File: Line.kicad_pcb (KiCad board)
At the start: 2 copper layers, 141 x 29 mm, 50 parts, among them U0 QRE1113GR, U1 QRE1113GR, U10 QRE1113GR, U11 QRE1113GR, U12 QRE1113GR, U13 QRE1113GR, U14 QRE1113GR, U16 CD74HC4067M, U2 QRE1113GR, U3 QRE1113GR, U4 QRE1113GR, U5 QRE1113GR, U6 QRE1113GR, U7 QRE1113GR, U8 QRE1113GR, U9 QRE1113GR

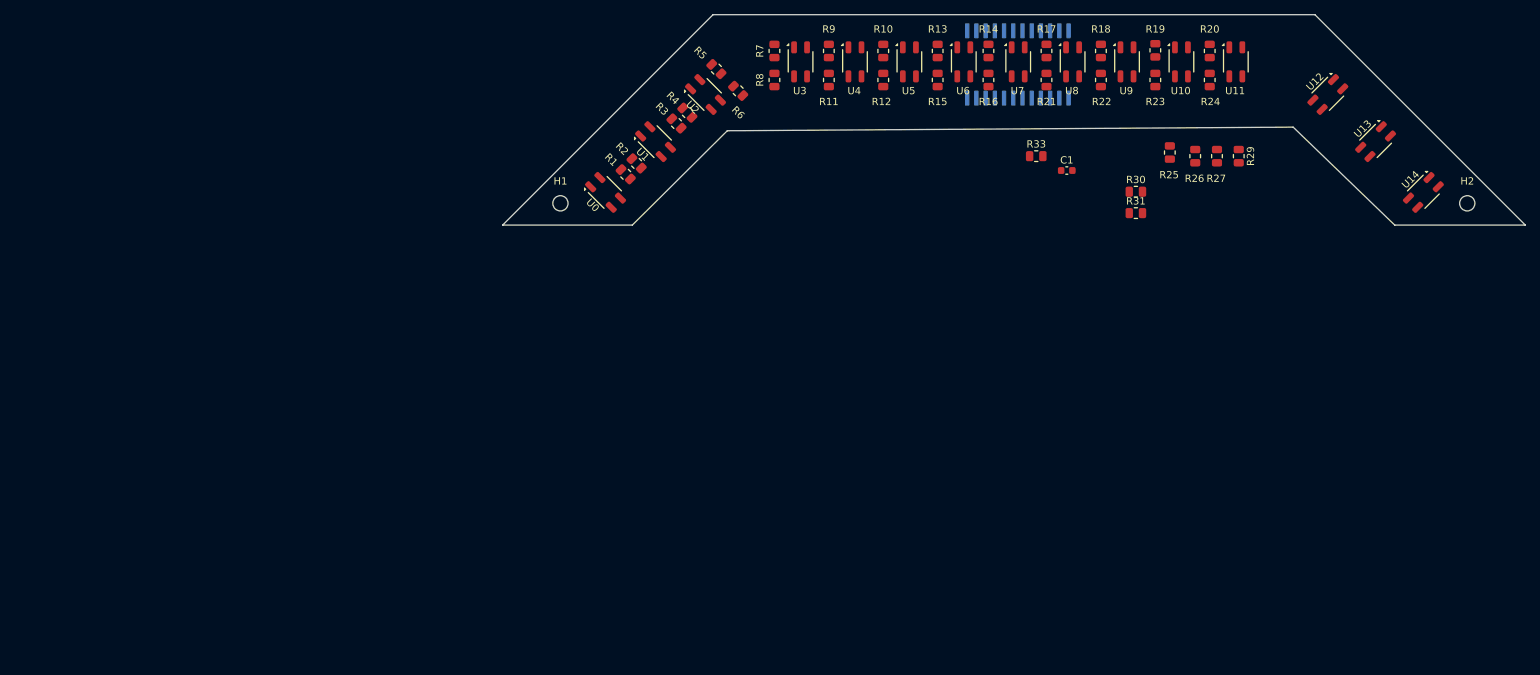
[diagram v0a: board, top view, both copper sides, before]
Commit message: sap route
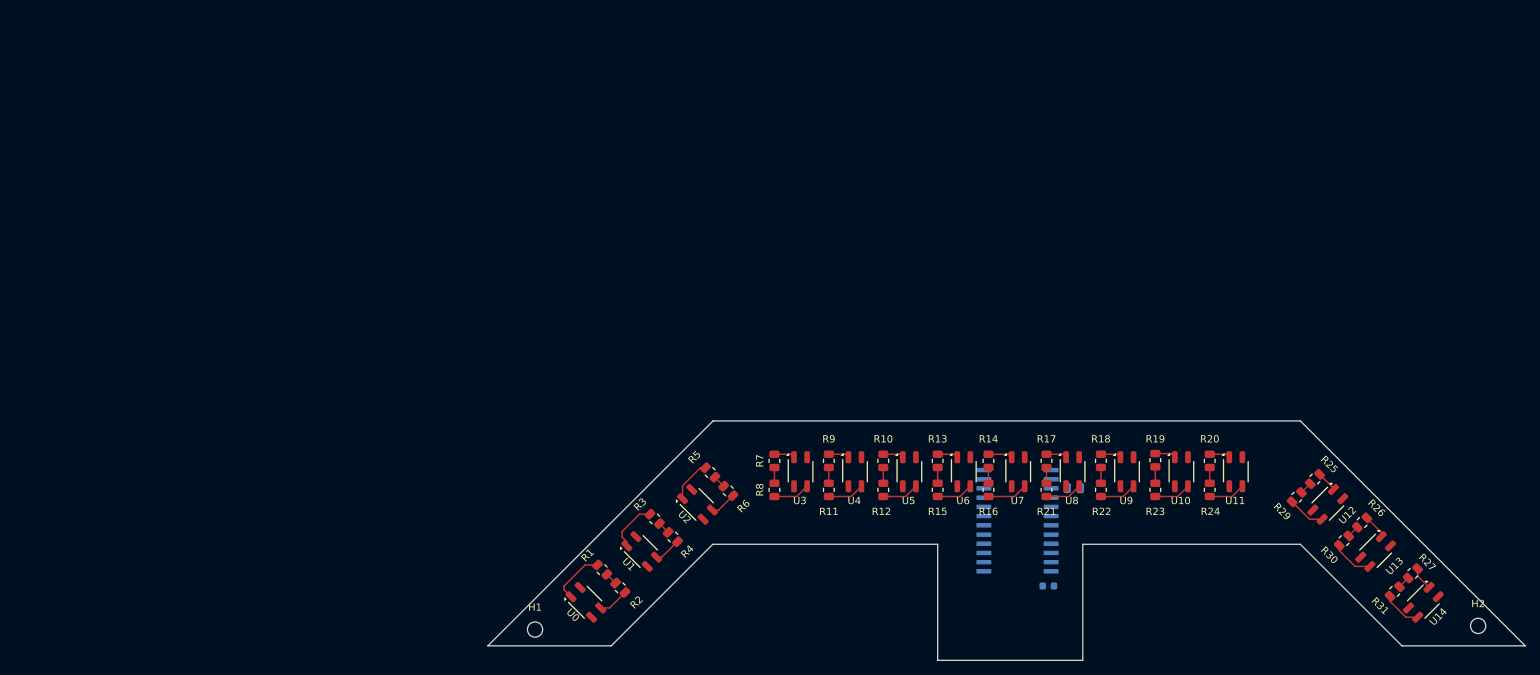
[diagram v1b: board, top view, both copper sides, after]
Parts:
- C1, R33: moved to B.Cu
- moved R27 63.5 mm to (267.0, 142.0), turned to 45 degrees
- moved R31 63.2 mm to (264.5, 144.5), turned to -135 degrees
- moved U16 62.9 mm to (212.5, 134.8), turned to 0 degrees
- moved H1 58.9 mm to (146.0, 149.8)
- moved R2 58.5 mm to (157.8, 144.0), turned to -45 degrees
- moved R4 58.5 mm to (165.0, 137.0), turned to -45 degrees
- moved H2 58.3 mm to (276.0, 149.2)
- moved C1 57.3 mm to (216.8, 143.8), turned to 180 degrees
- moved U0 56.6 mm to (153.0, 146.0)
- moved U1 56.5 mm to (160.7, 139.0)
- moved U2 56.5 mm to (168.4, 132.5)
- moved R10 56.5 mm to (194.0, 126.5)
- moved R11 56.5 mm to (186.5, 130.5)
- moved R12 56.5 mm to (194.0, 130.5)
- moved R13 56.5 mm to (201.5, 126.5)
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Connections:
- U1 pad 1: Net-(U0-A) -> Net-(U1-A)
- U1 pad 3: C0 -> C1
- U2 pad 1: Net-(U0-A) -> Net-(U2-A)
- U2 pad 3: C0 -> C2
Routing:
- net +3.3V: track 0.00 -> 30.0 mm
- net Net-(U0-A): track 0.00 -> 7.67 mm
- net Net-(U1-A): track 0.00 -> 7.09 mm
- net Net-(U2-A): track 0.00 -> 5.99 mm
- net C13: track 0.00 -> 5.85 mm
- net C7: track 0.00 -> 5.59 mm
- net C14: track 0.00 -> 5.44 mm
- net C12: track 0.00 -> 5.14 mm
- net C9: track 0.00 -> 5.09 mm
- net C8: track 0.00 -> 5.09 mm
- net C6: track 0.00 -> 5.09 mm
- net C5: track 0.00 -> 5.09 mm
- net C4: track 0.00 -> 5.09 mm
- net C3: track 0.00 -> 5.09 mm
- net C11: track 0.00 -> 5.09 mm
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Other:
- board size 141 x 29 mm -> 143 x 33 mm

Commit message: đon
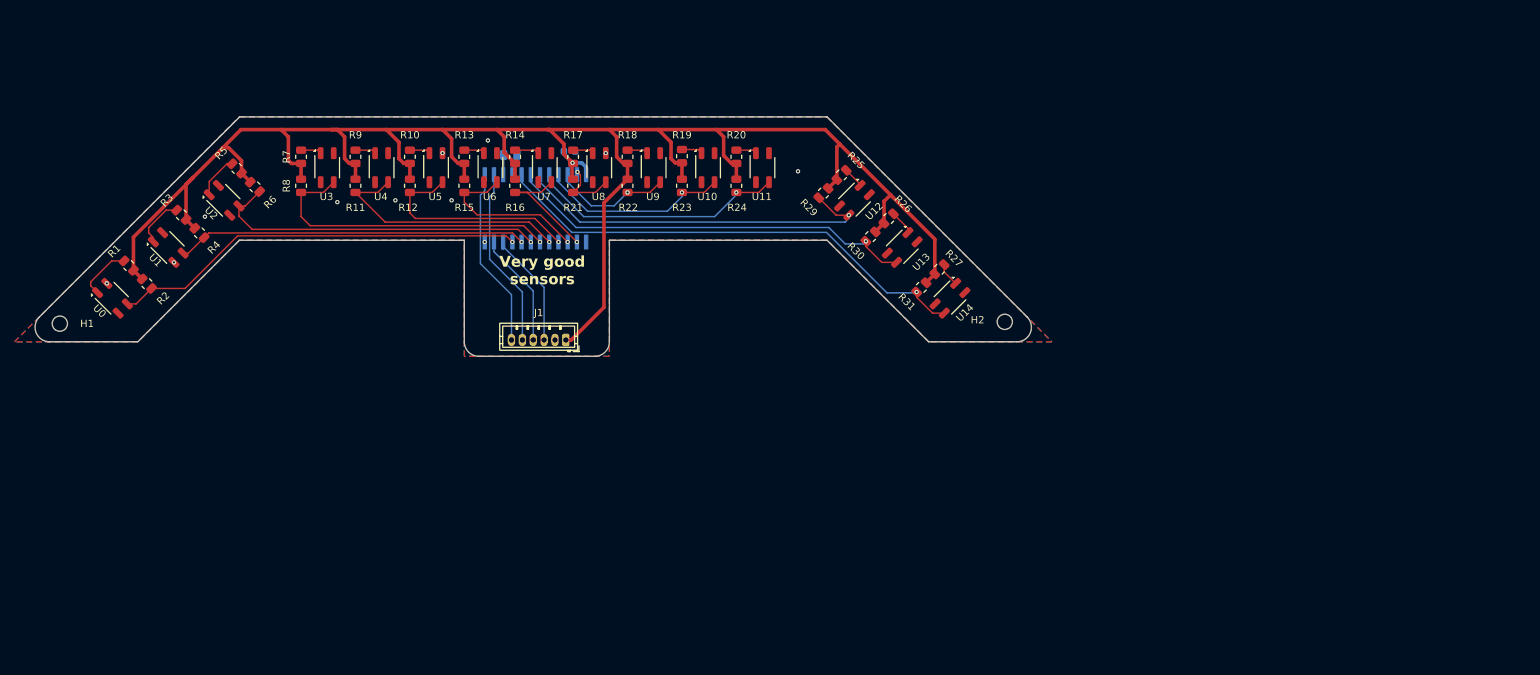
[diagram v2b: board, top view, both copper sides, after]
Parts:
- added J1: Conn_01x06_Pin, Connector_JST:JST_ZH_B6B-ZR_1x06_P1.50mm_Vertical, F.Cu at (150.2, 109.8)
- moved R33 90.2 mm to (142.6, 84.3)
- moved C1 89.1 mm to (150.8, 83.8), turned to 0 degrees
- moved U16 79.2 mm to (146.1, 91.7), turned to 90 degrees
- moved H1 77.9 mm to (80.5, 107.6)
- moved R6 77.6 mm to (107.4, 88.7)
- moved R5 77.6 mm to (104.9, 86.2)
- moved U2 77.6 mm to (103.1, 90.6)
- moved H2 77.6 mm to (210.8, 107.3)
- moved R1 77.6 mm to (90.0, 99.6)
- moved R10 77.6 mm to (128.8, 84.6)
- moved R11 77.6 mm to (121.2, 88.6)
- moved R12 77.6 mm to (128.8, 88.6)
- moved R13 77.6 mm to (136.2, 84.6)
- moved R14 77.6 mm to (143.2, 84.6)
- moved R15 77.6 mm to (136.2, 88.6)
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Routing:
- net +3.3V: track 30.0 -> 272.5 mm, vias 0 -> 1
- net C14: track 5.44 -> 67.3 mm, vias 0 -> 1
- net C0: track 4.23 -> 57.3 mm, vias 0 -> 1
- net C13: track 5.85 -> 56.7 mm, vias 0 -> 1
- net C12: track 5.14 -> 51.7 mm, vias 0 -> 1
- net C1: track 3.78 -> 48.3 mm, vias 0 -> 1
- net C2: track 3.67 -> 46.8 mm, vias 0 -> 1
- net C3: track 5.09 -> 42.8 mm, vias 0 -> 1
- net C11: track 5.09 -> 35.5 mm, vias 0 -> 1
- net C4: track 5.09 -> 34.6 mm, vias 0 -> 1
- net C5: track 5.09 -> 30.1 mm, vias 0 -> 1
- net S2: track 0.00 -> 24.9 mm
- net S3: track 0.00 -> 24.8 mm
- net C10: track 5.09 -> 26.2 mm, vias 0 -> 1
- net C6: track 5.09 -> 23.0 mm, vias 0 -> 1
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- added copper zone on B.Cu, net GND
- added copper zone on F.Cu, net GND
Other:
- board size 143 x 33 mm -> 137.3 x 33 mm
- board text added: "Very good sensors"
